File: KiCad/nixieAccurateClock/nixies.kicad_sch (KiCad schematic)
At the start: 7 parts, among them J10 Conn_02x05_Odd_Even

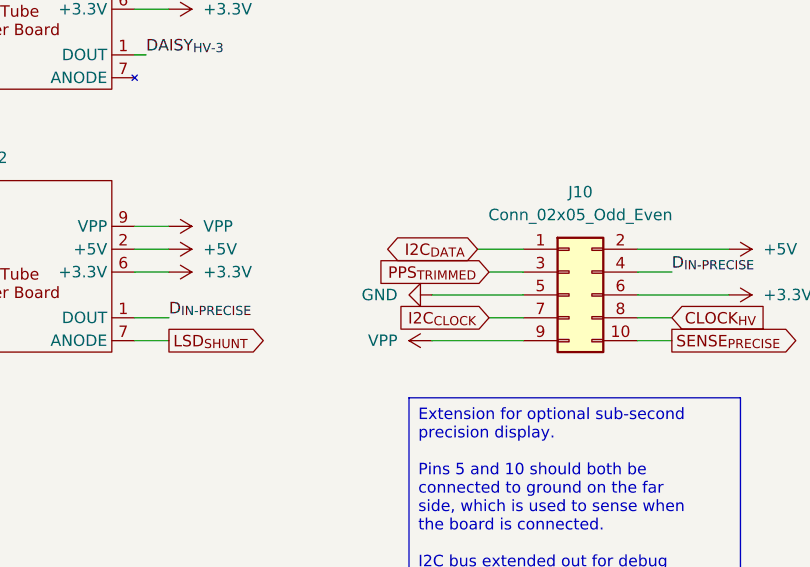
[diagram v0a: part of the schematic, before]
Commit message: DRC pass
it's messy
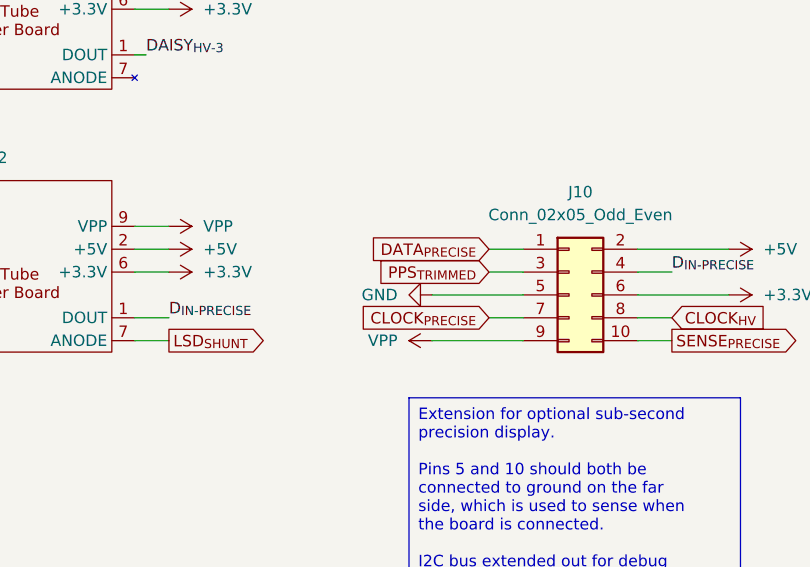
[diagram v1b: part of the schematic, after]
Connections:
- net I2C_{CLOCK} renamed CLOCK_{PRECISE}
- net I2C_{DATA} renamed DATA_{PRECISE}
